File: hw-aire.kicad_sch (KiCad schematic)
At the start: 53 parts, among them J1 Conn_01x02_Pin, J3 Screw_Terminal_01x12, J4 Conn_01x04_Pin, K1 JRC-21F(4100), K2 JRC-21F(4100), K3 JRC-21F(4100), Q1 PMBT3904235, Q2 PMBT3904235, Q3 PMBT3904235, Q5 PMBT3904235, SW1 SW_Push, SW2 SW_Push, U1 HLK-2M05, U2 NCP1117-3.3_SOT223, U3 ESP-12E, U4 SHT4x, U5 BMP581

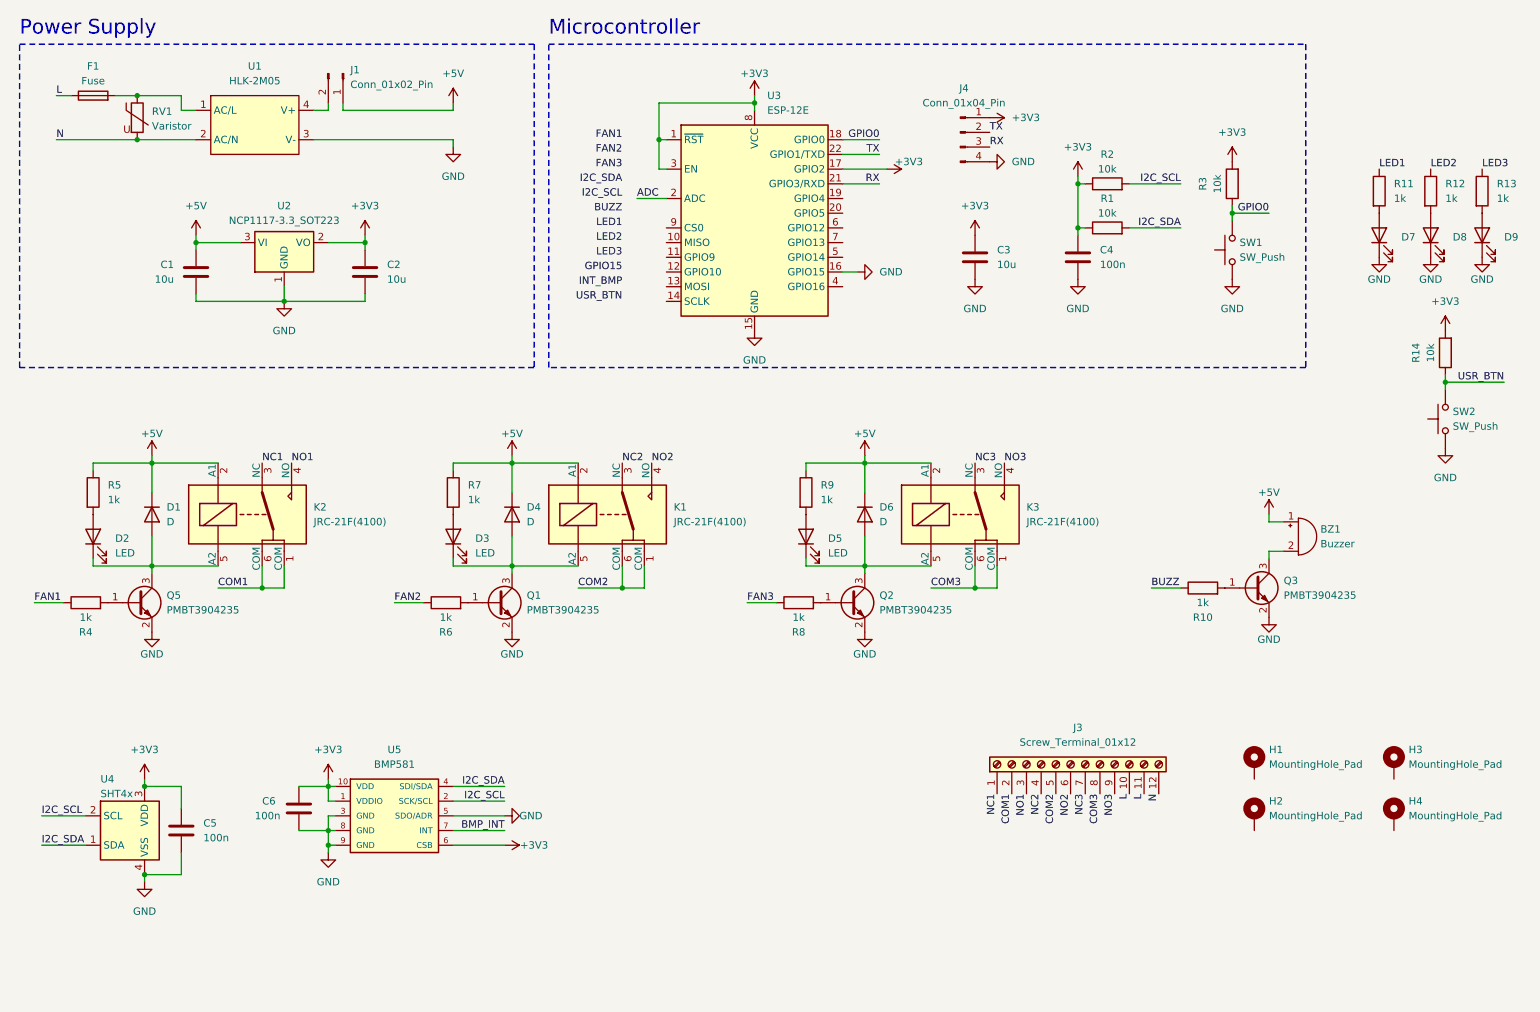
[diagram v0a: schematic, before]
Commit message: Update schematic
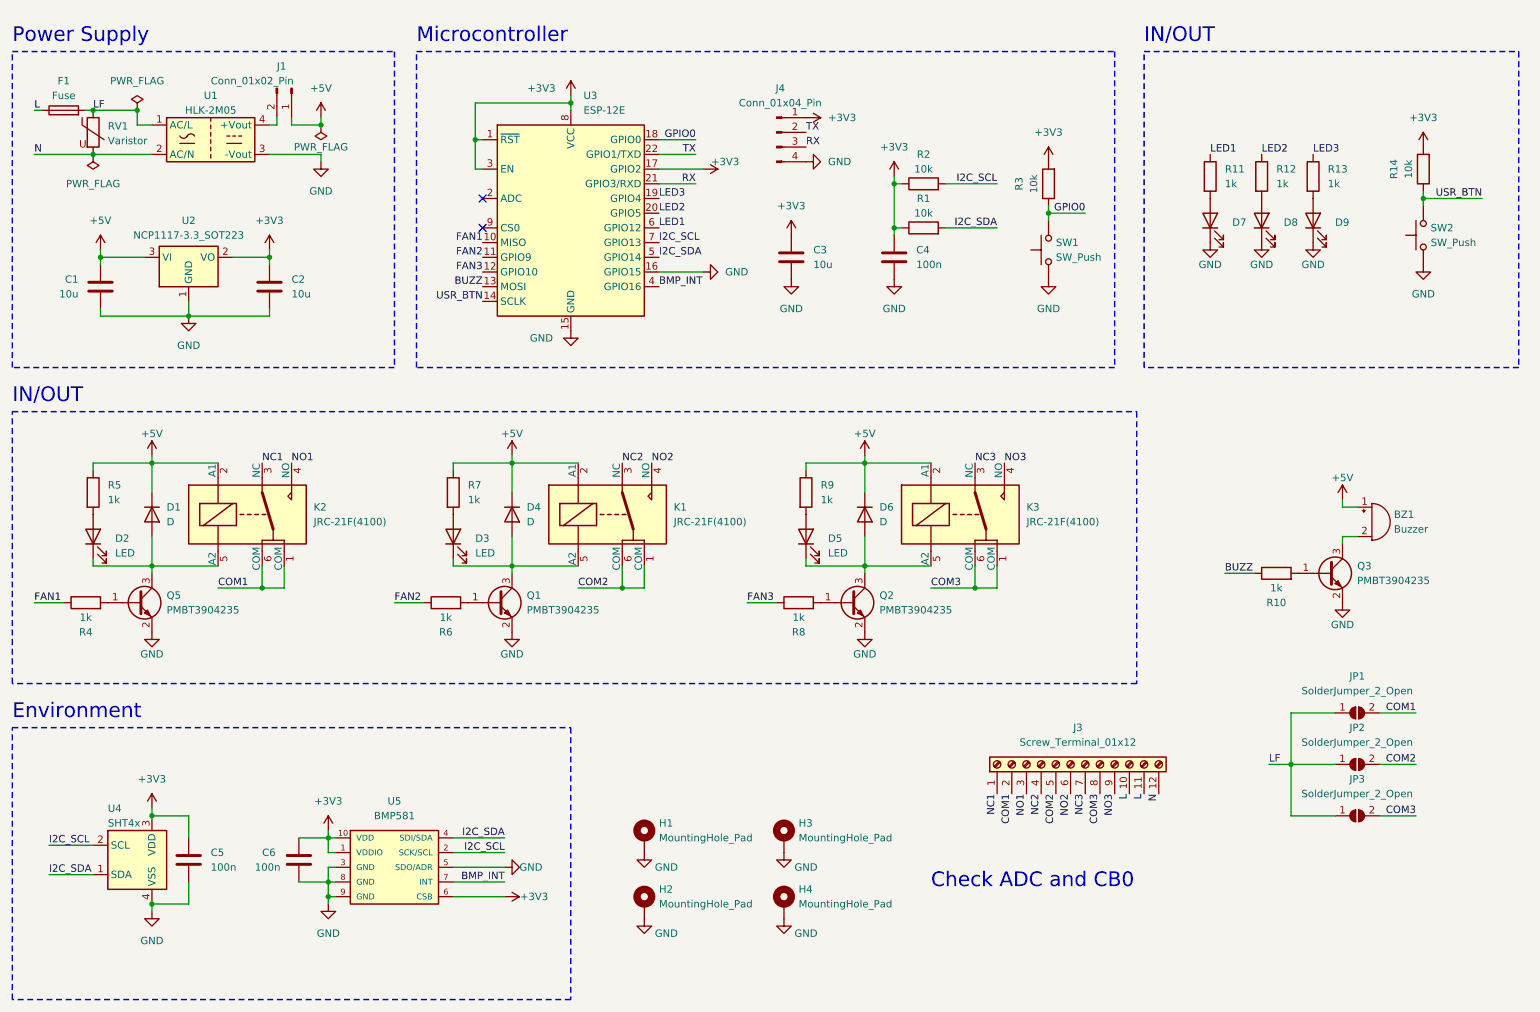
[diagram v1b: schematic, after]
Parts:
- added JP1, JP2, JP3: SolderJumper_2_Open, Jumper:SolderJumper-2_P1.3mm_Open_TrianglePad1.0x1.5mm, symbol Jumper:SolderJumper_2_Open
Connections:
- net BMP_INT: now also U3.4 (GPIO16)
- net BUZZ: now also U3.13 (MOSI)
- net COM1: now also JP1.2 (B)
- net COM2: now also JP2.2 (B)
- net COM3: now also JP3.2 (B)
- net FAN1: now also U3.10 (MISO)
- net FAN2: now also U3.11 (GPIO9)
- net FAN3: now also U3.12 (GPIO10)
- net GND: now also H1.1, H2.1, H3.1, H4.1
- net I2C_SCL: now also U3.7 (GPIO13)
- net I2C_SDA: now also U3.5 (GPIO14)
- net LED1: now also U3.6 (GPIO12)
- net LED2: now also U3.20 (GPIO5)
- net LED3: now also U3.19 (GPIO4)
- net USR_BTN: now also U3.14 (SCLK)
- net LF: now reaches F1.2, RV1.1, U1.1 (AC/L)
- net LF: now also JP1.1 (A), JP2.1 (A), JP3.1 (A)
- net ADC: no longer names the net of U3.2 (ADC)
- no-connect marks 0 -> 2
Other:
- note added: "Check ADC and CB0"
- note added: "Environment"
- note added: "IN/OUT"
- company: (none) -> Guillermo González
- title: (none) -> Aire
- moved on the sheet: BZ1, C1, C2, C3, C4, C5, C6, D7, D8, D9, F1, H1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
